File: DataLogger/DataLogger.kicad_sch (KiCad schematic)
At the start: 25 parts, among them U1 24LC1025, U2 24LC1025, U3 DS1337, U4 ATMEGA328P-AU, Y1 Crystal, Y2 Crystal

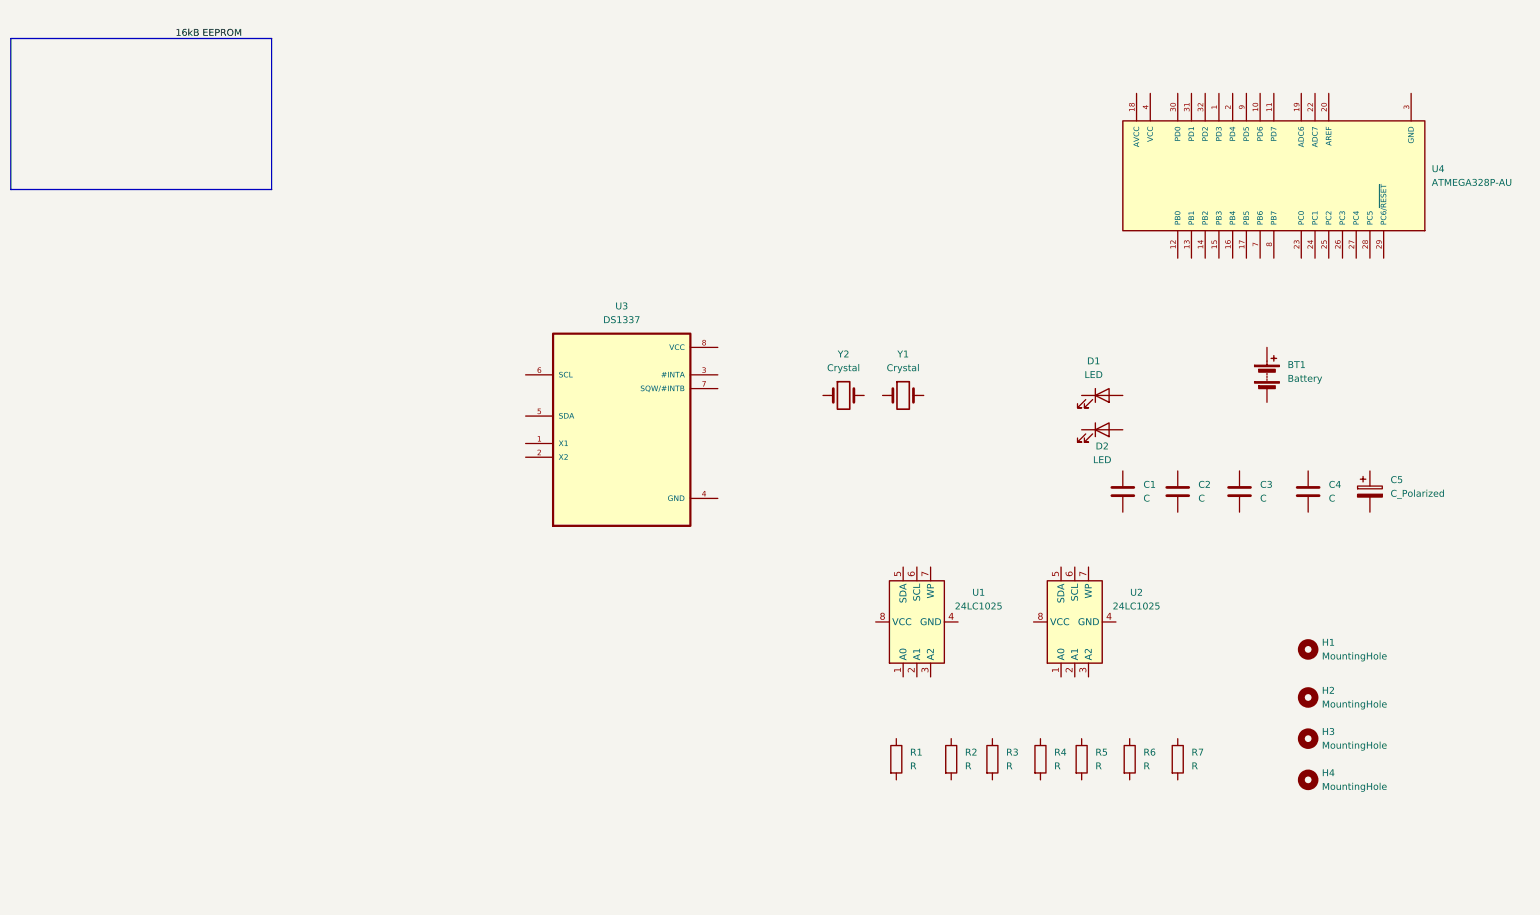
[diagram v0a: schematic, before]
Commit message: more
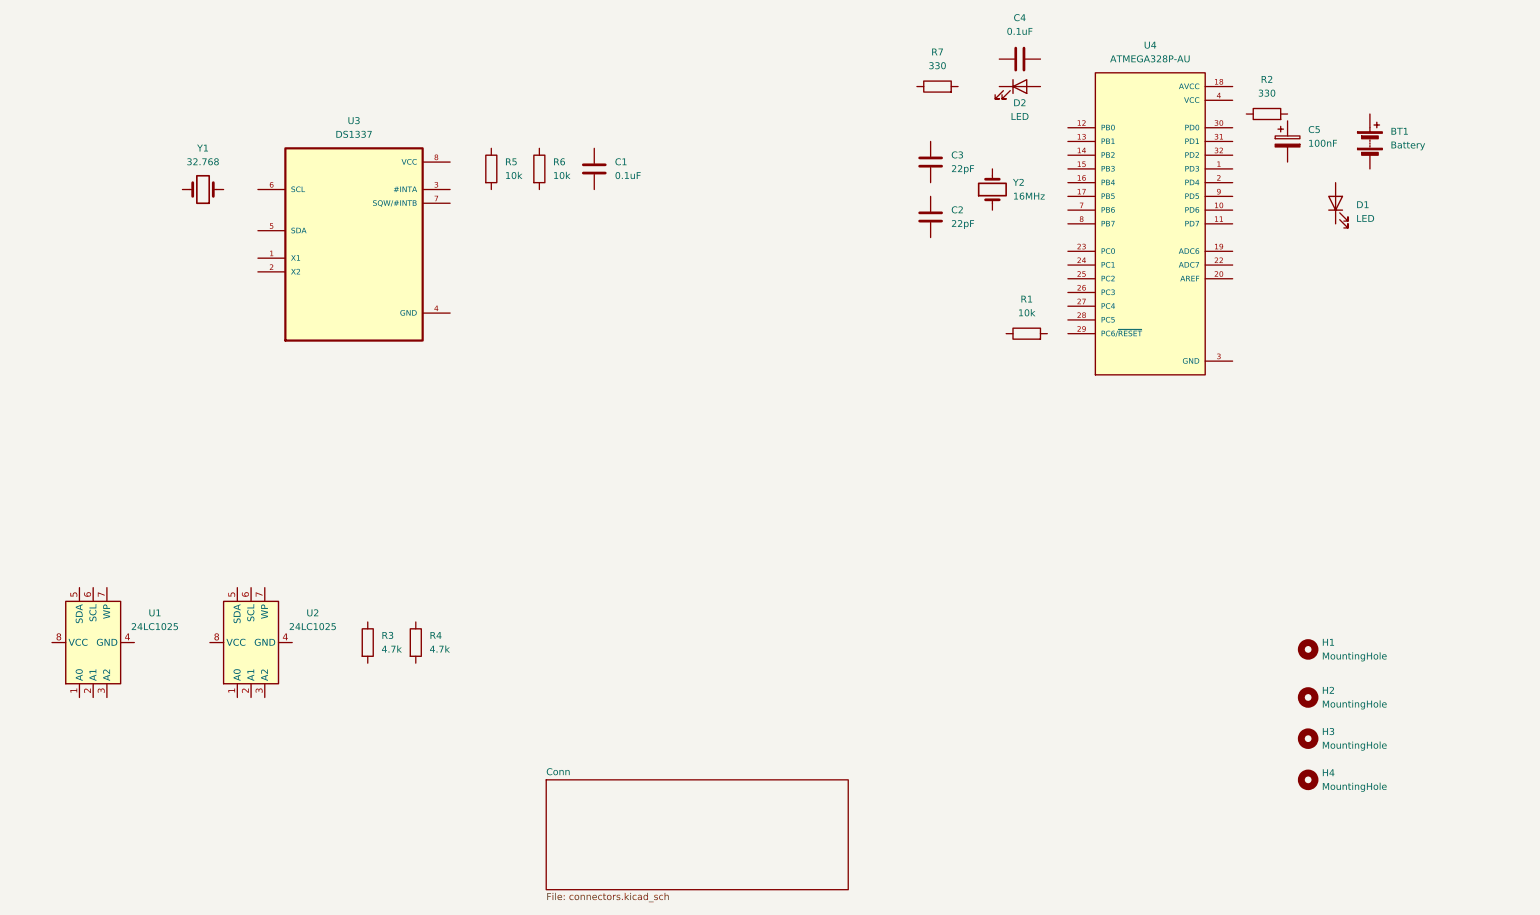
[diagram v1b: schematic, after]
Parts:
- C1, C4: value C -> 0.1uF
- C2, C3: value C -> 22pF
- C5: value C_Polarized -> 100nF
- R1, R5, R6: value R -> 10k
- R2, R7: value R -> 330
- R3, R4: value R -> 4.7k
- Y1: value Crystal -> 32.768
- Y2: value Crystal -> 16MHz
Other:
- added sheet Conn (connectors.kicad_sch)
- moved on the sheet: BT1, C1, C2, C3, C4, C5, D1, D2, R1, R2, R3, R4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
